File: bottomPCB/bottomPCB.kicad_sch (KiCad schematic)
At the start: 34 parts, among them P1 Pfostenstecker_8_2x4, U1 ESP32-WROOM-32, U2 Pfostenstecker_6_2x3, U3 Switch, U4 Pinhead_1x02H, U5 Pinhead_1x02H, U6 AKKU 1, U7 AKKU 2, U8 LM1117IMPX-3_3_NOPB, U9 LM1117IMPX-3_3_NOPB

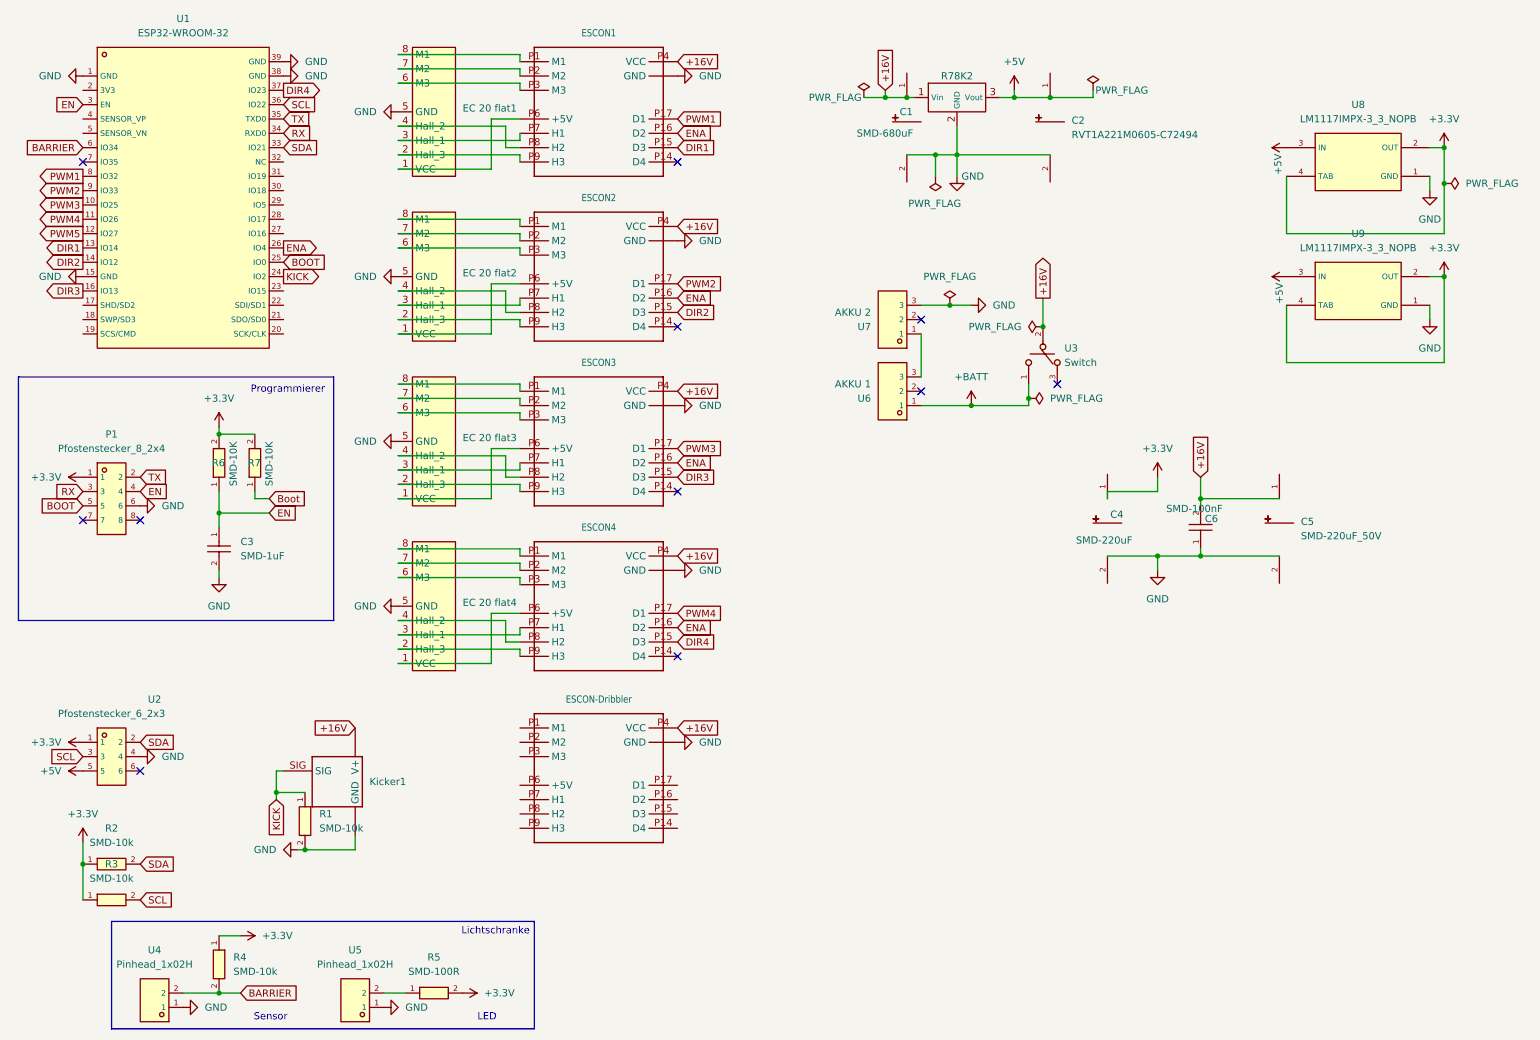
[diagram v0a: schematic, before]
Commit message: added comments
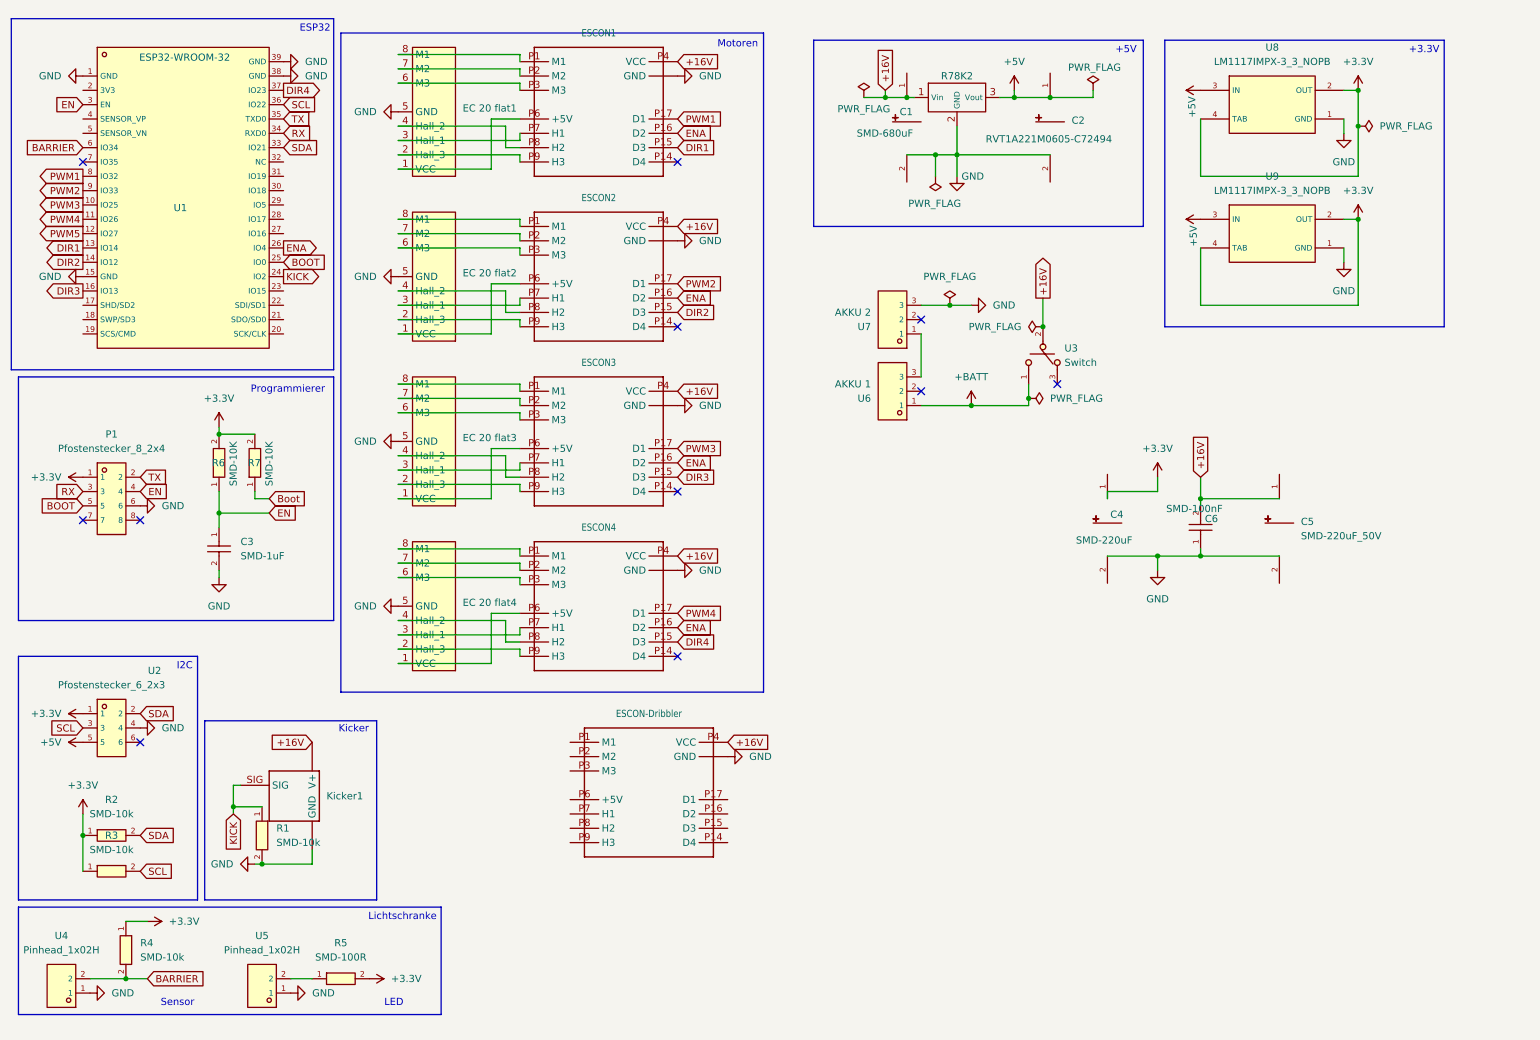
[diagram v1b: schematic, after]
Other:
- note added: "+3.3V"
- note added: "+5V"
- note added: "ESP32"
- note added: "I2C"
- note added: "Kicker"
- note added: "Motoren"
- moved on the sheet: ESCON-Dribbler, Kicker1, R1, R2, R3, R4, R5, U2, U4, U5, U8, U9
